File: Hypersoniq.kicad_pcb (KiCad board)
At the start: 4 copper layers, 40.4 x 100 mm, 138 parts, among them J1 Conn_01x10_Pin, J2 Conn_01x10_Pin, J3 Conn_01x10_Pin, J4 Eurorack_10_pin_power, U1 TL074, U2 SSI2140, U3 SSI2140, U4 SSI2140, U5 SSI2140, U6 TL072

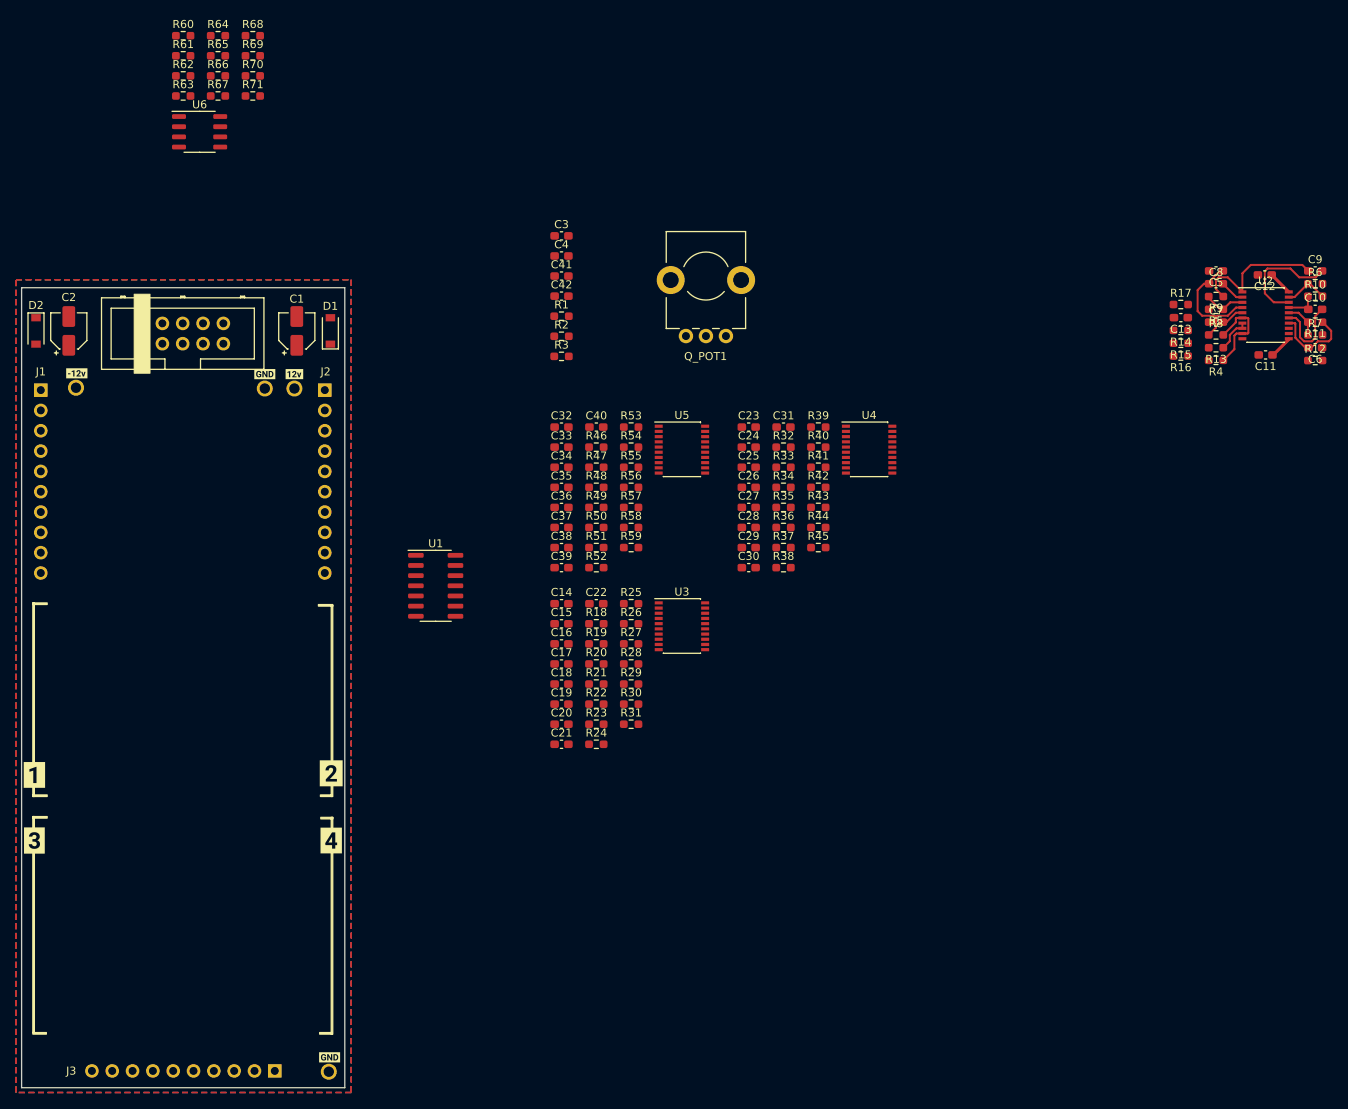
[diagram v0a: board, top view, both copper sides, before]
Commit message: Revert "Revert "PCB Layout""
This reverts commit 17ea893c43406ccb0184a474adf0eed468bf1595.
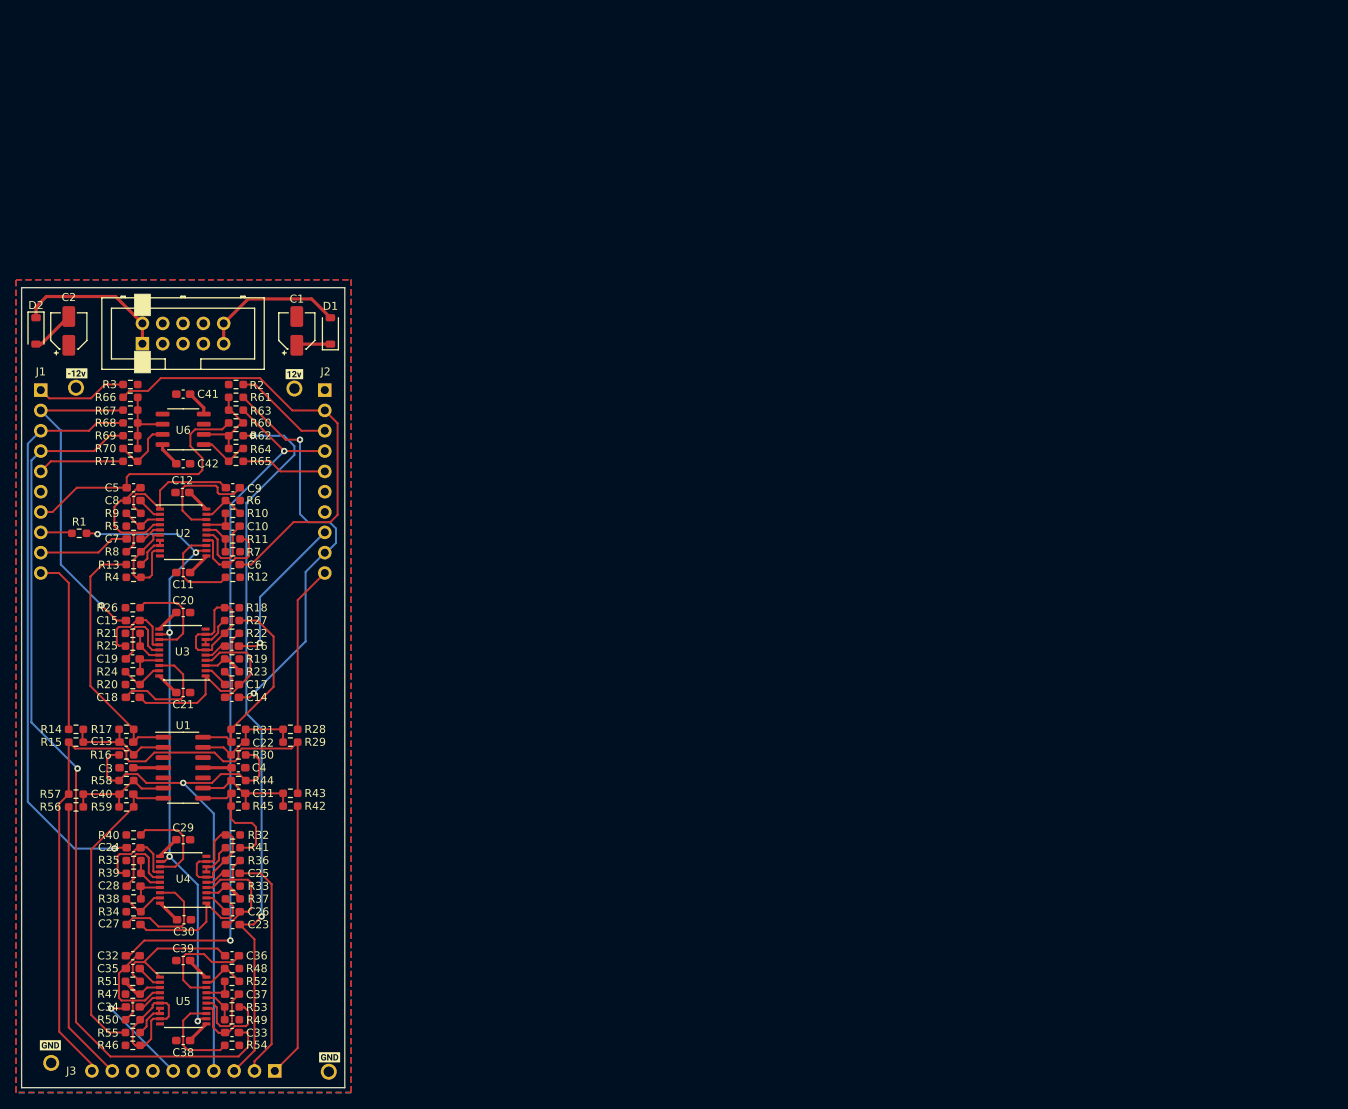
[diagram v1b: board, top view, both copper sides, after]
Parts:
- removed Q_POT1: 10k, Custom_Footprints:Alpha_9mm_Potentiometer_Aligned
- removed kibuzzard-63F9EC4B: G***, kibuzzard-63F9EC4B
- removed kibuzzard-63F9ECEE: G***, kibuzzard-63F9ECEE
- removed kibuzzard-63FCE890: G***, kibuzzard-63FCE890
- removed kibuzzard-63FCEF0D: G***, kibuzzard-63FCEF0D
- moved R14 146.8 mm to (56.8, 105.2)
- moved R15 146.8 mm to (56.8, 106.8)
- moved R17 142.1 mm to (63.1, 105.2), turned to 180 degrees
- moved C13 142.1 mm to (63.1, 106.8), turned to 0 degrees
- moved R16 140.9 mm to (63.1, 108.4)
- moved C11 138.0 mm to (70.2, 85.6)
- moved C12 138.0 mm to (70.1, 75.6)
- moved U2 138.0 mm to (70.2, 80.6)
- moved R10 138.0 mm to (76.4, 78.2)
- moved R4 138.0 mm to (64.0, 86.2)
- moved C5 138.0 mm to (64.0, 75.0)
- moved C7 138.0 mm to (64.0, 81.4)
- moved C8 138.0 mm to (64.0, 76.6)
- moved R13 138.0 mm to (64.0, 84.6)
- moved R5 138.0 mm to (64.0, 79.8)
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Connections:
- C22 pad 1: Net-(U1B--) -> Net-(U1D--)
- C40 pad 1: Net-(U1D--) -> Net-(U1B--)
- J1 pad 1: /FREQ_POT_VH -> /FREQ_POT_VL
- J1 pad 10: /AUDIO_IN2 -> /FREQ_CV1
- J1 pad 3: /4POLE_OUT4 -> /4POLE_OUT3
- J1 pad 4: /FREQ_POT_VL -> /4POLE_OUT4
- J1 pad 5: /FREQ_POT -> /AUDIO_MIX_4POLE
- J1 pad 7: /FREQ_CV1 -> /1POLE_OUT1
- J1 pad 9: /AUDIO_MIX -> /AUDIO_IN1
- J2 pad 3: /4POLE_OUT3 -> /FREQ_POT_VH
- J2 pad 5: GND -> /AUDIO_MIX_1POLE
- J2 pad 8: /AUDIO_IN1 -> /AUDIO_IN2
- J3 pad 1: /AUDIO_IN3 -> /FREQ_CV3
- J3 pad 10: /FREQ_CV3 -> /FREQ_JACK
- J3 pad 2: /FREQ_CV4 -> /AUDIO_IN3
- J3 pad 3: /1POLE_OUT1 -> /1POLE_OUT3
- J3 pad 4: GND -> /FREQ_POT
- J3 pad 5: /AUDIO_IN4 -> GND
- J3 pad 6: GND -> /AUDIO_IN4
- J3 pad 8: /FREQ_JACK -> GND
- J3 pad 9: /1POLE_OUT3 -> /FREQ_CV4
- R28 pad 1: Net-(U1B--) -> Net-(U1D--)
- R29 pad 1: Net-(U1B--) -> Net-(U1D--)
- R30 pad 1: Net-(U1B--) -> Net-(U1D--)
- R31 pad 2: Net-(U1B--) -> Net-(U1D--)
- R56 pad 1: Net-(U1D--) -> Net-(U1B--)
- R57 pad 1: Net-(U1D--) -> Net-(U1B--)
- R58 pad 1: Net-(U1D--) -> Net-(U1B--)
- R59 pad 2: Net-(U1D--) -> Net-(U1B--)
- R65 pad 2: /AUDIO_MIX -> /AUDIO_MIX_1POLE
- R71 pad 2: /AUDIO_MIX -> /AUDIO_MIX_4POLE
- U1 pad 14: /Filter_Voice4/FREQ_CONTROL -> /Filter_Voice2/FREQ_CONTROL
- U1 pad 7: /Filter_Voice2/FREQ_CONTROL -> /Filter_Voice4/FREQ_CONTROL
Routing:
- net /4POLE_OUT4: track 0.00 -> 112.1 mm, vias 0 -> 1
- net /1POLE_OUT3: track 0.00 -> 92.3 mm, vias 0 -> 2
- net /1POLE_OUT4: track 0.00 -> 90.1 mm, vias 0 -> 2
- net /FREQ_JACK: track 0.00 -> 82.1 mm
- net /Q_CONTROL: track 0.00 -> 81.5 mm, vias 0 -> 5
- net /4POLE_OUT3: track 0.00 -> 72.6 mm, vias 0 -> 1
- net /FREQ_POT: track 0.00 -> 66.4 mm, vias 0 -> 1
- net /4POLE_OUT1: track 0.00 -> 56.4 mm
- net /1POLE_OUT2: track 0.00 -> 50.9 mm, vias 0 -> 2
- net /4POLE_OUT2: track 0.00 -> 41.6 mm, vias 0 -> 1
- net /Filter_Voice4/FREQ_CONTROL: track 0.00 -> 39.0 mm
- net /FREQ_CV4: track 0.00 -> 35.3 mm
- net /FREQ_CV3: track 0.00 -> 34.3 mm
- net /1POLE_OUT1: track 0.00 -> 33.6 mm
- net /Filter_Voice1/FREQ_CONTROL: track 0.00 -> 32.1 mm
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
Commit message: Revert "PCB Layout"
This reverts commit f9e64c4088f3b37948fb3949196b7229d7a48ca0.
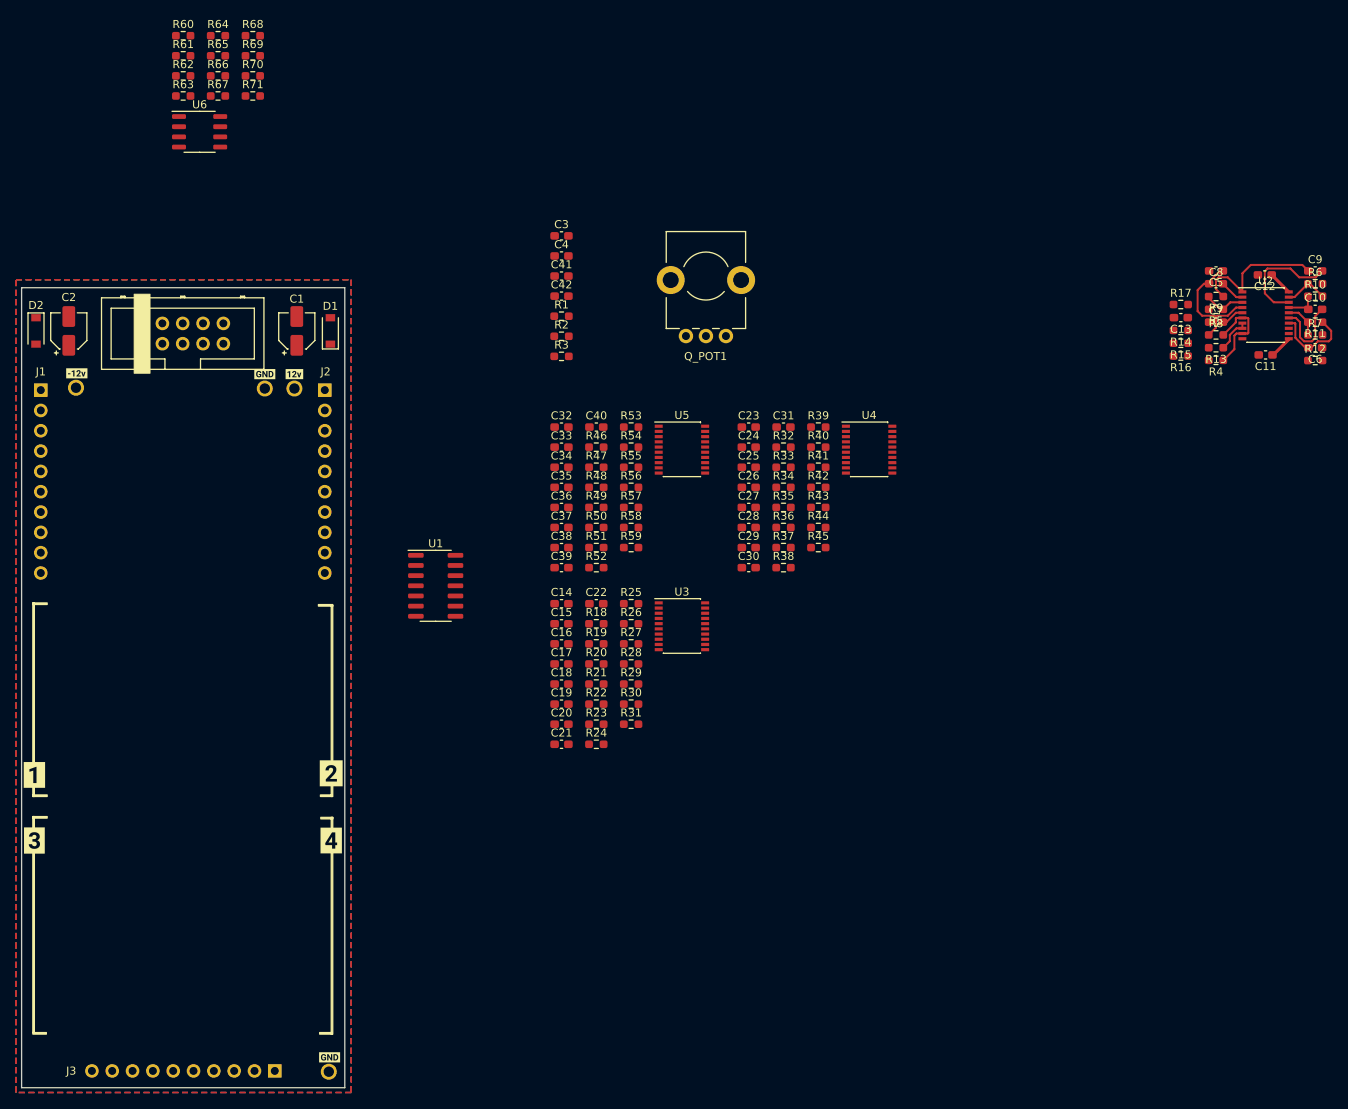
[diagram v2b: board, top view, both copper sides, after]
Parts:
- added Q_POT1: 10k, Custom_Footprints:Alpha_9mm_Potentiometer_Aligned, F.Cu at (135.5, 48.5)
- added kibuzzard-63F9EC4B: G***, kibuzzard-63F9EC4B, F.Cu at (51.6, 119.1)
- added kibuzzard-63F9ECEE: G***, kibuzzard-63F9ECEE, F.Cu at (88.7, 119.1)
- added kibuzzard-63FCE890: G***, kibuzzard-63FCE890, F.Cu at (51.6, 110.9)
- added kibuzzard-63FCEF0D: G***, kibuzzard-63FCEF0D, F.Cu at (88.7, 110.7)
- moved R14 146.8 mm to (194.9, 55.3)
- moved R15 146.8 mm to (194.9, 56.9)
- moved R17 142.1 mm to (194.9, 52.1), turned to 0 degrees
- moved C13 142.1 mm to (194.9, 53.7), turned to 180 degrees
- moved R16 140.9 mm to (194.9, 58.5)
- moved C11 138.0 mm to (205.5, 58.4)
- moved C12 138.0 mm to (205.4, 48.4)
- moved U2 138.0 mm to (205.5, 53.5)
- moved R10 138.0 mm to (211.7, 51.1)
- moved R4 138.0 mm to (199.3, 59.1)
- moved C5 138.0 mm to (199.3, 47.9)
- moved C7 138.0 mm to (199.3, 54.3)
- moved C8 138.0 mm to (199.3, 49.5)
- moved R13 138.0 mm to (199.3, 57.5)
- moved R5 138.0 mm to (199.3, 52.7)
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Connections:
- C22 pad 1: Net-(U1D--) -> Net-(U1B--)
- C40 pad 1: Net-(U1B--) -> Net-(U1D--)
- J1 pad 1: /FREQ_POT_VL -> /FREQ_POT_VH
- J1 pad 10: /FREQ_CV1 -> /AUDIO_IN2
- J1 pad 3: /4POLE_OUT3 -> /4POLE_OUT4
- J1 pad 4: /4POLE_OUT4 -> /FREQ_POT_VL
- J1 pad 5: /AUDIO_MIX_4POLE -> /FREQ_POT
- J1 pad 7: /1POLE_OUT1 -> /FREQ_CV1
- J1 pad 9: /AUDIO_IN1 -> /AUDIO_MIX
- J2 pad 3: /FREQ_POT_VH -> /4POLE_OUT3
- J2 pad 5: /AUDIO_MIX_1POLE -> GND
- J2 pad 8: /AUDIO_IN2 -> /AUDIO_IN1
- J3 pad 1: /FREQ_CV3 -> /AUDIO_IN3
- J3 pad 10: /FREQ_JACK -> /FREQ_CV3
- J3 pad 2: /AUDIO_IN3 -> /FREQ_CV4
- J3 pad 3: /1POLE_OUT3 -> /1POLE_OUT1
- J3 pad 4: /FREQ_POT -> GND
- J3 pad 5: GND -> /AUDIO_IN4
- J3 pad 6: /AUDIO_IN4 -> GND
- J3 pad 8: GND -> /FREQ_JACK
- J3 pad 9: /FREQ_CV4 -> /1POLE_OUT3
- R28 pad 1: Net-(U1D--) -> Net-(U1B--)
- R29 pad 1: Net-(U1D--) -> Net-(U1B--)
- R30 pad 1: Net-(U1D--) -> Net-(U1B--)
- R31 pad 2: Net-(U1D--) -> Net-(U1B--)
- R56 pad 1: Net-(U1B--) -> Net-(U1D--)
- R57 pad 1: Net-(U1B--) -> Net-(U1D--)
- R58 pad 1: Net-(U1B--) -> Net-(U1D--)
- R59 pad 2: Net-(U1B--) -> Net-(U1D--)
- R65 pad 2: /AUDIO_MIX_1POLE -> /AUDIO_MIX
- R71 pad 2: /AUDIO_MIX_4POLE -> /AUDIO_MIX
- U1 pad 14: /Filter_Voice2/FREQ_CONTROL -> /Filter_Voice4/FREQ_CONTROL
- U1 pad 7: /Filter_Voice4/FREQ_CONTROL -> /Filter_Voice2/FREQ_CONTROL
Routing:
- net /4POLE_OUT4: track 112.1 -> 0.00 mm, vias 1 -> 0
- net /1POLE_OUT3: track 92.3 -> 0.00 mm, vias 2 -> 0
- net /1POLE_OUT4: track 90.1 -> 0.00 mm, vias 2 -> 0
- net /FREQ_JACK: track 82.1 -> 0.00 mm
- net /Q_CONTROL: track 81.5 -> 0.00 mm, vias 5 -> 0
- net /4POLE_OUT3: track 72.6 -> 0.00 mm, vias 1 -> 0
- net /FREQ_POT: track 66.4 -> 0.00 mm, vias 1 -> 0
- net /4POLE_OUT1: track 56.4 -> 0.00 mm
- net /1POLE_OUT2: track 50.9 -> 0.00 mm, vias 2 -> 0
- net /4POLE_OUT2: track 41.6 -> 0.00 mm, vias 1 -> 0
- net /Filter_Voice4/FREQ_CONTROL: track 39.0 -> 0.00 mm
- net /FREQ_CV4: track 35.3 -> 0.00 mm
- net /FREQ_CV3: track 34.3 -> 0.00 mm
- net /1POLE_OUT1: track 33.6 -> 0.00 mm
- net /Filter_Voice1/FREQ_CONTROL: track 32.1 -> 0.00 mm
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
